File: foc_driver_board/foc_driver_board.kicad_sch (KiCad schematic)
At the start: 42 parts, among them J1 STM32-Prog-Header, J2 Conn_01x14, J3 USB_C_Receptacle_USB2.0_14P, SW1 SW_Push, U1 Male Conn, U2 AZ1117IH-3.3, U3 AZ1117IH-5.0, U4 MCP2542FD, U5 STM32G491KEUx, U6 MCP6007, U7 USBLC6-2SC6, X1 OXETDLJANF-8MHZ

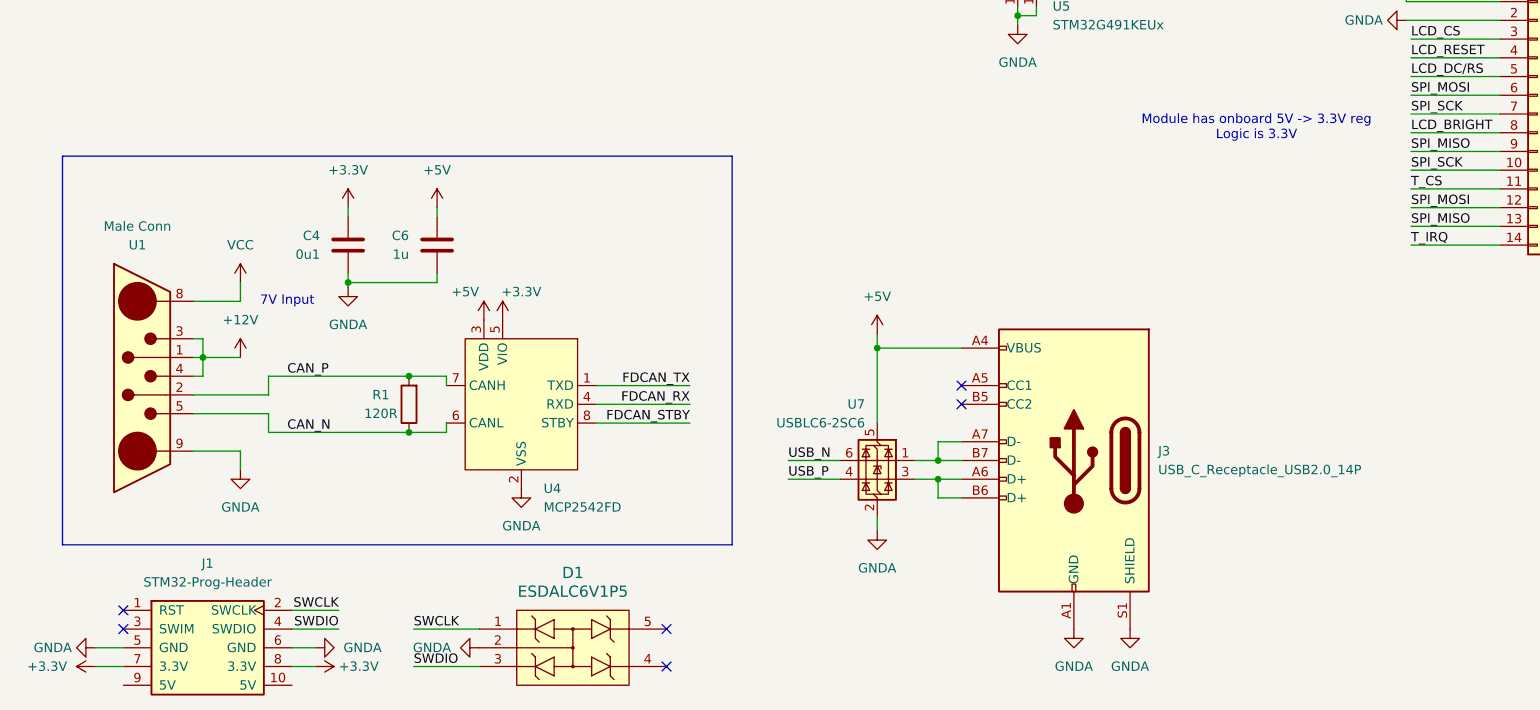
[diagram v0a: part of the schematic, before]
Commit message: $
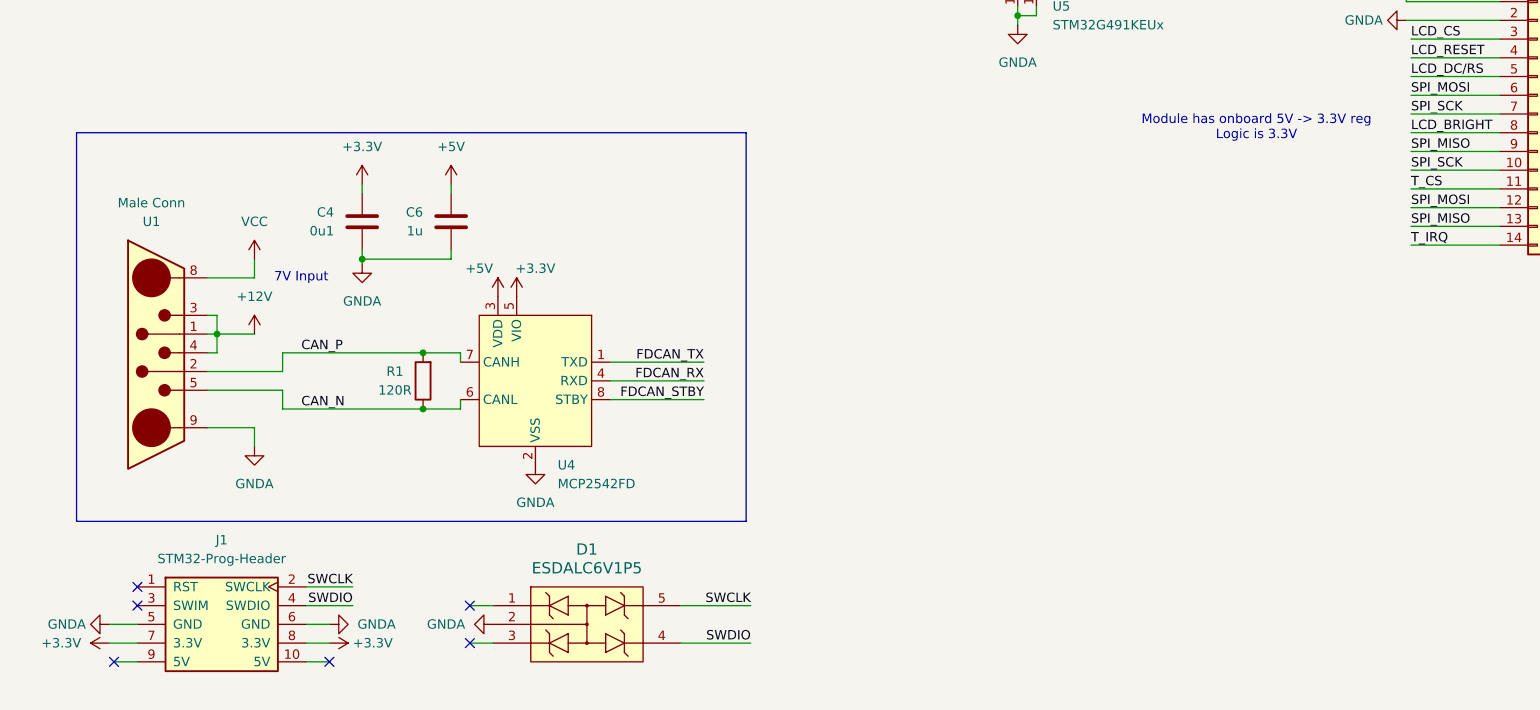
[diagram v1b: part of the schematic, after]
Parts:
- removed J3: USB_C_Receptacle_USB2.0_14P, Connector_USB:USB_C_Receptacle_GCT_USB4105-xx-A_16P_TopMnt_Horizontal, symbol Connector:USB_C_Receptacle_USB2.0_14P
- removed U7: USBLC6-2SC6, Package_TO_SOT_SMD:SOT-23-6, symbol Power_Protection:USBLC6-2SC6
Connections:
- net SWCLK: now also D1.5; no longer D1.1
- net SWDIO: now also D1.4; no longer D1.3
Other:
- moved on the sheet: C4, C6, D1, J1, R1, U1, U4
